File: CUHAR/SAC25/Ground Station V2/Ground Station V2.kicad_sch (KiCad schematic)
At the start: 6 parts, among them J1 SMA Connector, U1 ESP32-S3

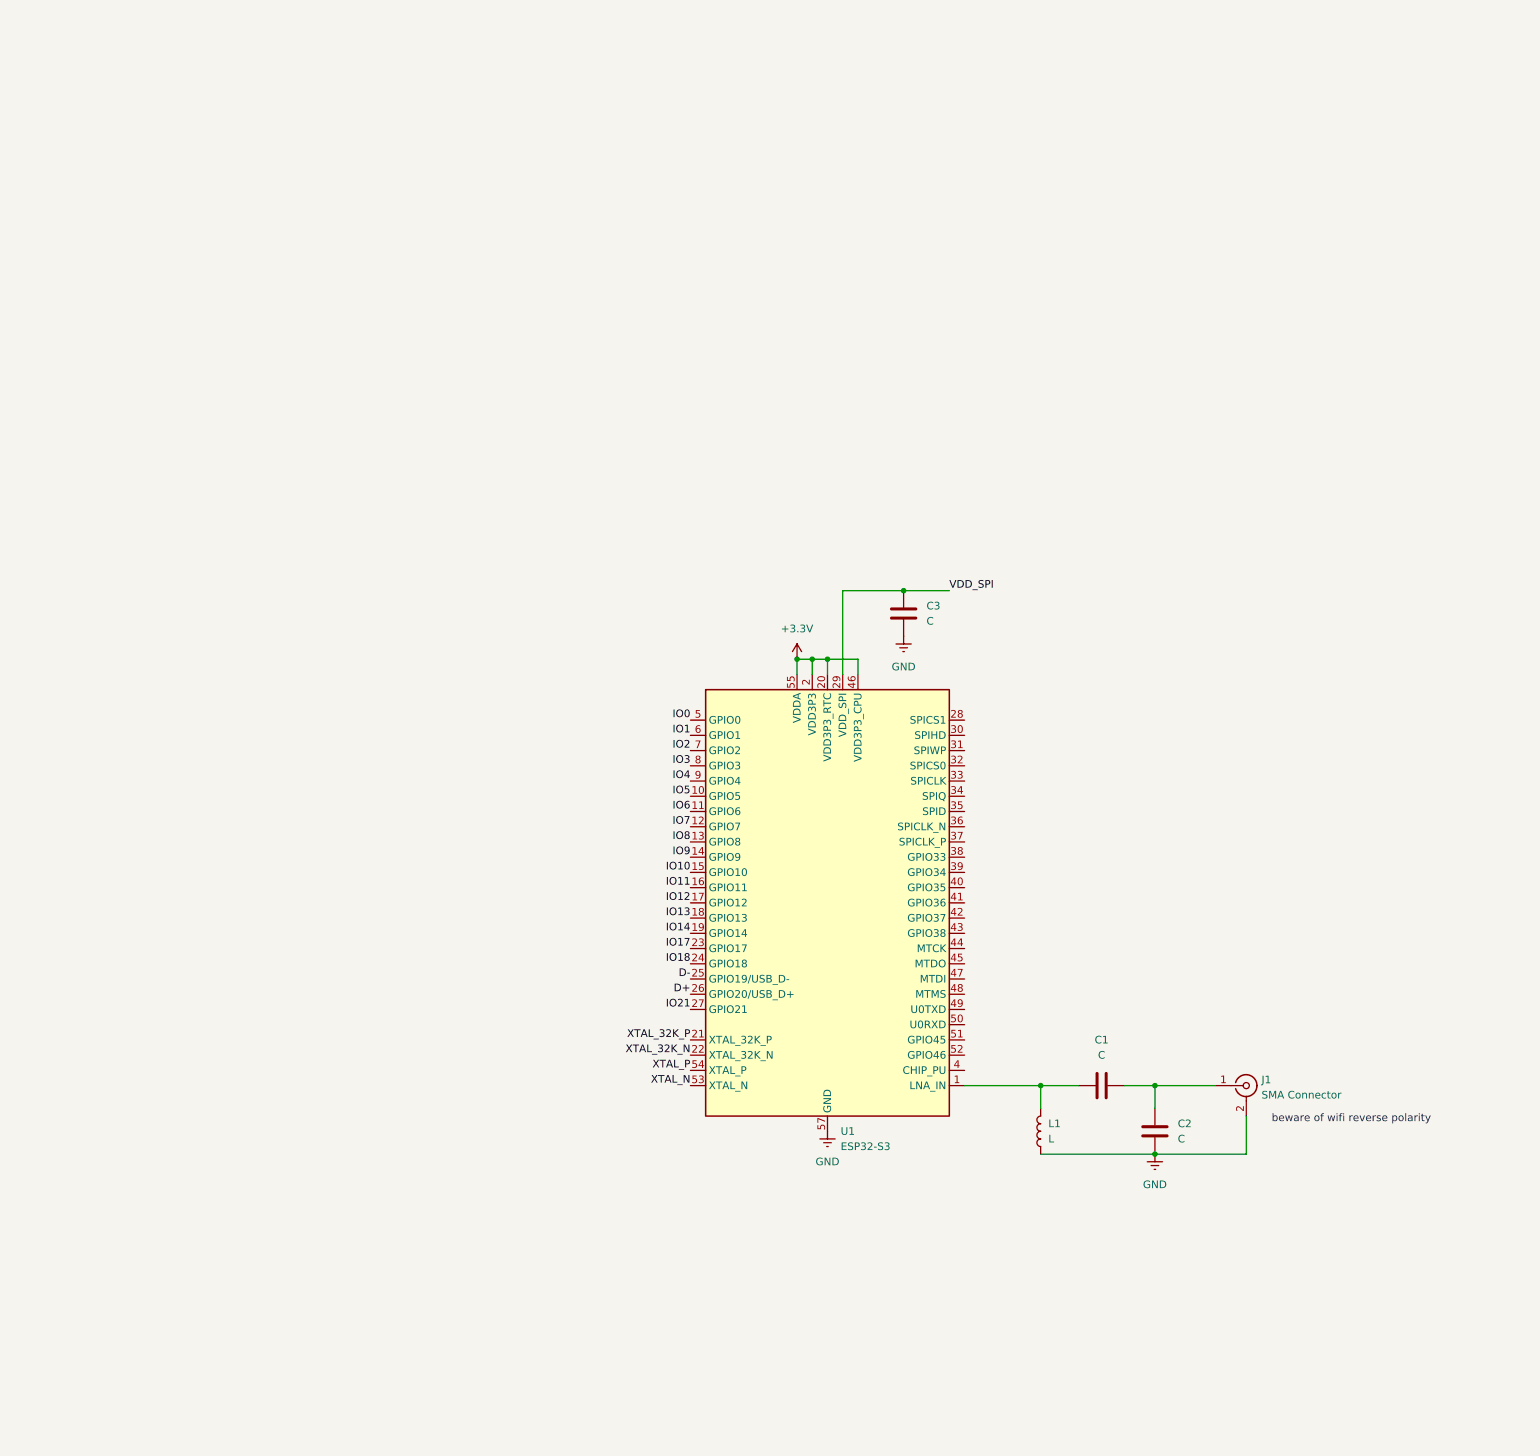
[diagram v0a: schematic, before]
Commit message: idk man
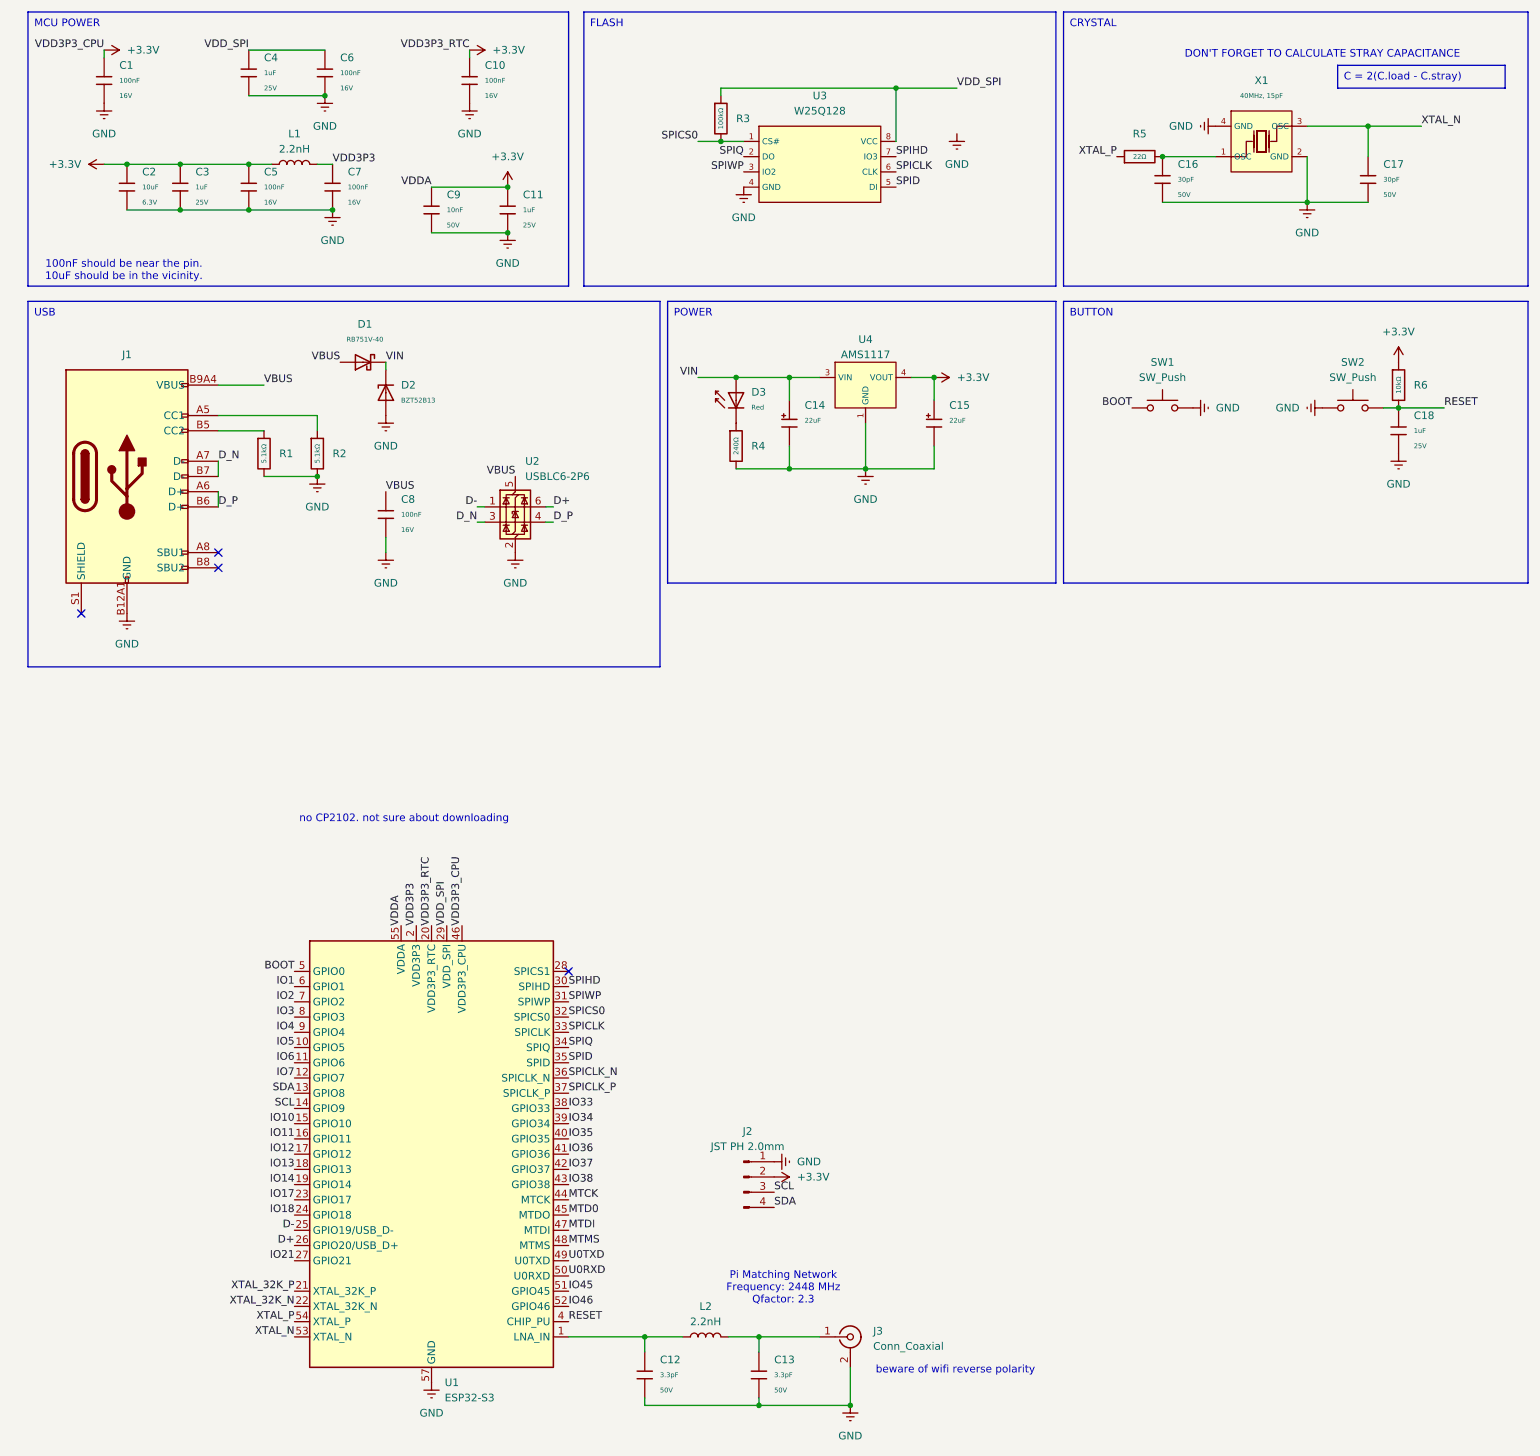
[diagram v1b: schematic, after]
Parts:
- removed C1, C2, C3: C, symbol Device:C
- removed J1: SMA Connector, symbol Connector:Conn_Coaxial
- removed U1: ESP32-S3, Package_DFN_QFN:QFN-56-1EP_7x7mm_P0.4mm_EP4x4mm, symbol MCU_Espressif:ESP32-S3
- added C1, C10, C5, C6, C7, C8: 100nF, JLCPCB-Kicad-Footprints:C_0402, symbol JLCPCB-Capacitors:0402,100nF
- added C11, C18, C3, C4: 1uF, JLCPCB-Kicad-Footprints:C_0402, symbol JLCPCB-Capacitors:0402,1uF
- added C12, C13: 3.3pF, JLCPCB-Kicad-Footprints:C_0402, symbol JLCPCB-Capacitors:0402,3.3pF
- added C14, C15: 22uF, JLCPCB-Kicad-Footprints:C_CASE-A-3216-18(mm), symbol JLCPCB-Capacitors:CASE-A-3216-18(mm),10uF
- added C16, C17: 30pF, JLCPCB-Kicad-Footprints:C_0402, symbol JLCPCB-Capacitors:0402,30pF
- added C2: 10uF, JLCPCB-Kicad-Footprints:C_0402, symbol JLCPCB-Capacitors:0402,10uF
- added C9: 10nF, JLCPCB-Kicad-Footprints:C_0402, symbol JLCPCB-Capacitors:0402,10nF
- added D1: RB751V-40, JLCPCB-Kicad-Footprints:D_SOD-323, symbol JLCPCB-Diodes:Schottky,RB751V-40
- added D2: BZT52B13, JLCPCB-Kicad-Footprints:D_SOD-123, symbol JLCPCB-Diodes:Zener,BZT52B13
- added D3: Red, JLCPCB-Kicad-Footprints:D_0603, symbol JLCPCB-Diodes:LED,0603,Red
- added J1: Connector, USB-TYPE-C-16P, JLCPCB-Kicad-Footprints:TYPE-C-SMD_HX-TYPE-C-16PIN, symbol JLCPCB-Extended:Connector, USB-TYPE-C-16P
- added J2: JST PH 2.0mm, Connector_JST:JST_EH_B4B-EH-A_1x04_P2.50mm_Vertical, symbol Connector:Conn_01x04_Pin
- added J3: Conn_Coaxial, Connector_Coaxial:SMA_Amphenol_132289_EdgeMount, symbol Connector:Conn_Coaxial
- added L2: 2.2nH, JLCPCB-Kicad-Footprints:L_0402, symbol Device:L
- added R1, R2: 5.1kΩ, JLCPCB-Kicad-Footprints:R_0402, symbol JLCPCB-Resistors:0402,5.1kΩ
- added R3: 100kΩ, JLCPCB-Kicad-Footprints:R_0402, symbol JLCPCB-Resistors:0402,100kΩ
- added R4: 240Ω, JLCPCB-Kicad-Footprints:R_0603, symbol JLCPCB-Resistors:0603,240Ω
- added R5: 22Ω, JLCPCB-Kicad-Footprints:R_0402, symbol JLCPCB-Resistors:0402,22Ω
- added R6: 10kΩ, JLCPCB-Kicad-Footprints:R_0402, symbol JLCPCB-Resistors:0402,10kΩ
- added SW1, SW2: SW_Push, Button_Switch_SMD:SW_Push_SPST_NO_Alps_SKRK, symbol Switch:SW_Push
- added U1: ESP32-S3, JLCPCB-Kicad-Footprints:QFN-56-1EP_7x7mm_P0.4mm_EP4x4mm_ThermalVias, symbol JLCPCB-Extended:MCU, ESP32-S3
- added U2: USBLC6-2P6, Package_TO_SOT_SMD:SOT-666, symbol Power_Protection:USBLC6-2P6
- added U3: W25Q128, JLCPCB-Kicad-Footprints:SOIC-8_L5.3-W5.3-P1.27-LS8.0-BL, symbol JLCPCB-Memory:16MByte, SPI
- added U4: AMS1117, JLCPCB-Kicad-Footprints:SOT-223-3_L6.5-W3.4-P2.30-LS7.0-BR, symbol JLCPCB-Power:LDO, 3.3V, 1A
- added X1: 40MHz, 15pF, JLCPCB-Kicad-Footprints:OSC-SMD_4P-L3.2-W2.5-BL_SIT8008BI, symbol JLCPCB-Extended:Crystal, 40MHz, 15pF
- L1: value L -> 2.2nH; footprint (none) -> JLCPCB-Kicad-Footprints:L_0402; JLCPCB Part # (none) -> C86061
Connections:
- net +3.3V: now also L1.1, C1.1, C10.1, C11.1, C15.1, C2.1, C3.1, C5.1, C9.1, J2.2 (Pin_2), R6.1, U1.20 (VDD3P3_RTC), U1.46 (VDD3P3_CPU), U1.55 (VDDA), U1.56 (VDDA), U4.2 (VOUT), U4.4 (VOUT)
- net D+: now also U1.26 (GPIO20/USB_D+), U2.6 (I/O1)
- net D-: now also U1.25 (GPIO19/USB_D-), U2.1 (I/O1)
- net GND: now also C1.2, C10.2, C11.2, C12.2, C13.2, C14.2, C15.2, C16.2, C17.2, C18.2, C2.2, C3.2, C4.2, C5.2, C6.2, C7.2, C8.2, C9.2, D2.2, J1.A12B1 (GND), J1.B12A1 (GND), J2.1 (Pin_1), J3.2 (Ext), R1.2, R2.2, R4.2, SW1.2, SW2.1, U1.57 (GND), U2.2 (GND), U3.4 (GND), U4.1 (GND), X1.2 (GND), X1.4 (GND); no longer L1.1
- net IO1: now also U1.6 (GPIO1)
- net IO10: now also U1.15 (GPIO10)
- net IO11: now also U1.16 (GPIO11)
- net IO12: now also U1.17 (GPIO12)
- net IO13: now also U1.18 (GPIO13)
- net IO14: now also U1.19 (GPIO14)
- net IO17: now also U1.23 (GPIO17)
- net IO18: now also U1.24 (GPIO18)
- net IO2: now also U1.7 (GPIO2)
- net IO21: now also U1.27 (GPIO21)
- net IO3: now also U1.8 (GPIO3)
- net IO4: now also U1.9 (GPIO4)
- net IO5: now also U1.10 (GPIO5)
- net IO6: now also U1.11 (GPIO6)
- net IO7: now also U1.12 (GPIO7)
- net VDD_SPI: now also C4.1, C6.1, R3.1, U1.29 (VDD_SPI), U3.8 (VCC)
- net XTAL_32K_N: now also U1.22 (XTAL_32K_N)
- net XTAL_32K_P: now also U1.21 (XTAL_32K_P)
- net XTAL_N: now also C17.1, U1.53 (XTAL_N), X1.3 (OSC)
- net XTAL_P: now also R5.1, U1.54 (XTAL_P)
- net VDD3P3: now reaches L1.2
- net VDD3P3: now also C7.1, U1.2 (VDD3P3), U1.3 (VDD3P3)
- new net: C12.1, L2.1, U1.1 (LNA_IN)
- new net: C13.1, J3.1 (In), L2.2
- new net: J1.A5 (CC1), R2.1
- new net: J1.B5 (CC2), R1.1
- new net: C16.1, R5.2, X1.1 (OSC)
- new net: D3.1, R4.1
- new net BOOT: SW1.1, U1.5 (GPIO0)
- new net D_N: J1.A7 (D-), J1.B7 (D-), U2.3 (I/O2)
- new net D_P: J1.A6 (D+), J1.B6 (D+), U2.4 (I/O2)
- new net IO33: U1.38 (GPIO33)
- new net IO34: U1.39 (GPIO34)
- new net IO35: U1.40 (GPIO35)
- new net IO36: U1.41 (GPIO36)
- new net IO37: U1.42 (GPIO37)
- new net IO38: U1.43 (GPIO38)
- new net IO45: U1.51 (GPIO45)
- new net IO46: U1.52 (GPIO46)
- new net MTCK: U1.44 (MTCK)
- new net MTD0: U1.45 (MTDO)
- new net MTDI: U1.47 (MTDI)
- new net MTMS: U1.48 (MTMS)
- new net RESET: C18.1, R6.2, SW2.2, U1.4 (CHIP_PU)
- new net SCL: J2.3 (Pin_3), U1.14 (GPIO9)
- new net SDA: J2.4 (Pin_4), U1.13 (GPIO8)
- new net SPICLK: U1.33 (SPICLK), U3.6 (CLK)
- new net SPICLK_N: U1.36 (SPICLK_N)
- new net SPICLK_P: U1.37 (SPICLK_P)
- new net SPICS0: R3.2, U1.32 (SPICS0), U3.1 (CS#)
- new net SPID: U1.35 (SPID), U3.5 (DI)
- new net SPIHD: U1.30 (SPIHD), U3.7 (IO3)
- new net SPIQ: U1.34 (SPIQ), U3.2 (DO)
- new net SPIWP: U1.31 (SPIWP), U3.3 (IO2)
- new net U0RXD: U1.50 (U0RXD)
- new net U0TXD: U1.49 (U0TXD)
- new net VBUS: C8.1, D1.2, J1.A9B4 (VBUS), J1.B9A4 (VBUS), U2.5 (VBUS)
- new net VIN: C14.1, D1.1, D2.1, D3.2, U4.3 (VIN)
- no-connect marks 0 -> 4
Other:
- note added: "100nF should be near the pin. 10uF should be in the vicinity."
- note added: "DON'T FORGET TO CALCULATE STRAY CAPACITANCE"
- note added: "Pi Matching Network Frequency: 2448 MHz Qfactor: 2.3"
- note added: "no CP2102. not sure about downloading"
